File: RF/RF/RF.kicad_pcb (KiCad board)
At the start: 4 copper layers, 72.5 x 72.5 mm, 90 parts, among them IC201 CC1110F16RHHR, IC401 PE4250MLI-Z, IC501 RFFM6406SR, IC701 23K256-I_SN, IC702 SST25VF512A-33-4C-SAE, J101 Conn_Coaxial, J201 Conn_01x02, J601 Conn_01x02, J602 Conn_01x06, J603 Conn_02x05_Odd_Even, J801 ESQ-110-13-G-D, U301 0433BM15A0001, Y201 TG2520SMN 27.000M-MCGNNM3

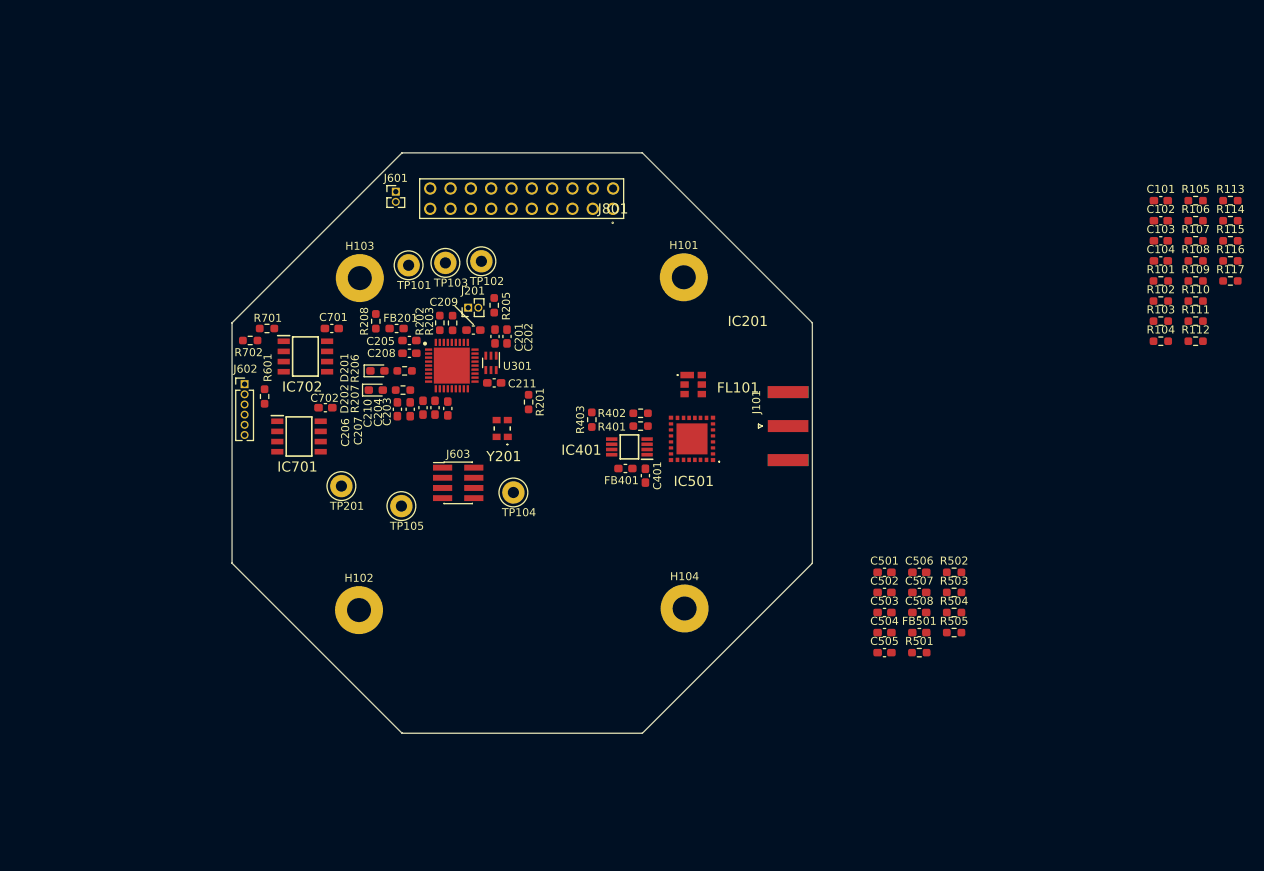
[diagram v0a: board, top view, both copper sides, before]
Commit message: layout rev 1.0
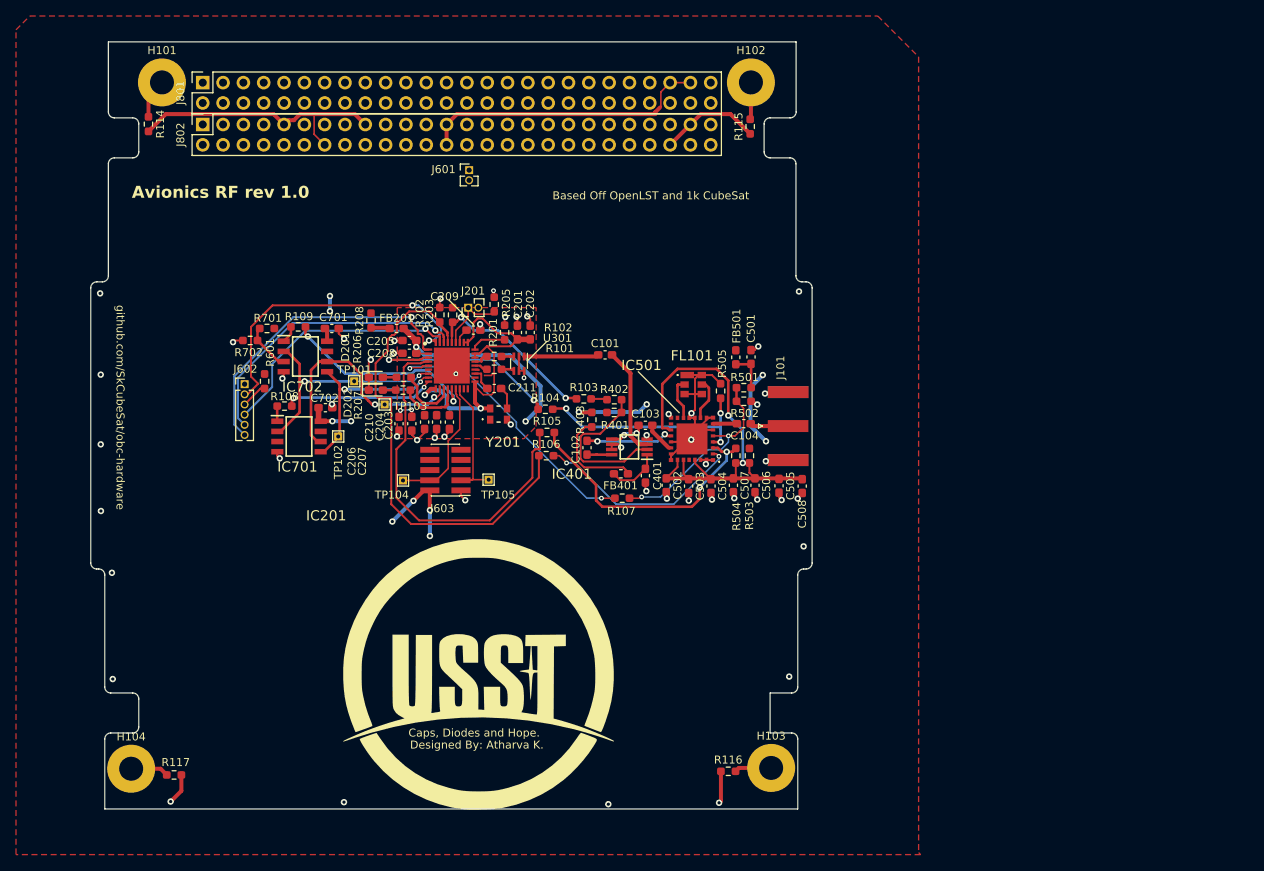
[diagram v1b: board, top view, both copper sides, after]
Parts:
- removed R110, R111, R112, R113: 0R, Resistor_SMD:R_0603_1608Metric_Pad0.98x0.95mm_HandSolder
- removed TP201: CC_SOC_2, TestPoint:TestPoint_Loop_D3.50mm_Drill1.4mm_Beaded
- added G***: LOGO, USST_logo:USST_logo, F.Cu at (108.5, 145.2)
- added G***: LOGO, USST_logo:USST_logo, B.Cu at (196.4, 139.0)
- added G***: LOGO, USST_logo:USST_logo, B.Cu at (207.5, 116.0)
- added G***: LOGO, USST_logo:USST_logo, B.Cu at (116.0, 116.7)
- added J802: Conn_02x26_Odd_Even, Connector_PinSocket_2.54mm:PinSocket_2x26_P2.54mm_Vertical, F.Cu at (74.1, 76.4)
- J603: footprint Connector_PinHeader_1.27mm:PinHeader_2x04_P1.27mm_Vertical_SMD -> Connector_PinHeader_1.27mm:PinHeader_2x05_P1.27mm_Vertical_SMD
- J801: value ESQ-110-13-G-D -> Conn_02x26_Odd_Even; footprint SamacSys_Parts:ESQ-110-Y-X-D -> Connector_PinSocket_2.54mm:PinSocket_2x26_P2.54mm_Vertical
- TP101, TP102, TP103, TP104, TP105: footprint TestPoint:TestPoint_Loop_D3.50mm_Drill1.4mm_Beaded -> TestPoint:TestPoint_THTPad_1.0x1.0mm_Drill0.5mm
- moved R117 145.8 mm to (70.5, 157.7), turned to 180 degrees
- moved R114 135.8 mm to (67.3, 76.4), turned to 90 degrees
- moved R108 115.3 mm to (84.3, 111.6), turned to 180 degrees
- moved R109 112.3 mm to (86.0, 101.7), turned to 180 degrees
- moved R116 89.5 mm to (139.8, 157.3)
- moved R106 86.3 mm to (117.0, 117.8)
- moved R105 86.1 mm to (117.1, 114.9)
- moved R101 84.1 mm to (110.5, 107.0)
- moved R102 83.6 mm to (110.5, 105.4)
- moved H102 82.2 mm to (142.6, 71.1)
- moved H103 80.0 mm to (145.1, 156.8)
- moved R107 78.6 mm to (126.5, 123.1)
- moved R104 77.4 mm to (116.9, 112.0)
- moved C102 77.1 mm to (122.1, 116.8), turned to 90 degrees
- moved R103 72.8 mm to (121.7, 110.7)
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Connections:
- IC201 pad 20: Net-(IC201-XOSC_Q2) -> unconnected-(IC201-XOSC_Q2-Pad20)
- J602 pad 2: /Connectors/UART0_RTS -> /CC1110/UART0_RTS
- J602 pad 4: /Connectors/UART0_RX -> /CC1110/UART0_RX
- J602 pad 5: /Connectors/UART0_TX -> /CC1110/UART0_TX
- J602 pad 6: /Connectors/UART0_CTS -> /CC1110/UART0_CTS
- J801 pad 1: /Standard Connector/GPIO_6 -> unconnected-(J801-Pin_1-Pad1)
- J801 pad 10: +5V -> unconnected-(J801-Pin_10-Pad10)
- J801 pad 11: /Standard Connector/GPIO_1 -> unconnected-(J801-Pin_11-Pad11)
- J801 pad 12: GND -> unconnected-(J801-Pin_12-Pad12)
- J801 pad 13: GND -> unconnected-(J801-Pin_13-Pad13)
- J801 pad 14: +3.3V -> unconnected-(J801-Pin_14-Pad14)
- J801 pad 15: /Standard Connector/CANL -> unconnected-(J801-Pin_15-Pad15)
- J801 pad 16: GND -> unconnected-(J801-Pin_16-Pad16)
- J801 pad 17: /Standard Connector/CANH -> unconnected-(J801-Pin_17-Pad17)
- J801 pad 18: +3.3V -> unconnected-(J801-Pin_18-Pad18)
- J801 pad 19: GND -> unconnected-(J801-Pin_19-Pad19)
- J801 pad 2: VBUS -> unconnected-(J801-Pin_2-Pad2)
- J801 pad 20: GND -> unconnected-(J801-Pin_20-Pad20)
- J801 pad 3: /Standard Connector/GPIO_5 -> unconnected-(J801-Pin_3-Pad3)
- J801 pad 4: GND -> unconnected-(J801-Pin_4-Pad4)
- J801 pad 5: /Standard Connector/GPIO_4 -> unconnected-(J801-Pin_5-Pad5)
- J801 pad 6: +5V -> unconnected-(J801-Pin_6-Pad6)
- J801 pad 7: /Standard Connector/GPIO_3 -> unconnected-(J801-Pin_7-Pad7)
- J801 pad 8: GND -> unconnected-(J801-Pin_8-Pad8)
- J801 pad 9: /Standard Connector/GPIO_2 -> unconnected-(J801-Pin_9-Pad9)
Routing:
- net GND: track 0.00 -> 135.8 mm, vias 0 -> 54
- net +3.3VA: track 0.00 -> 77.0 mm, vias 0 -> 6
- net Net-(IC501-VCC_RX): track 0.00 -> 70.8 mm, vias 0 -> 2
- net /CC1110/LST_TX_MODE: track 0.00 -> 59.7 mm
- net /CC1110/RF_EN: track 0.00 -> 47.0 mm
- net +3.3V: track 0.00 -> 41.5 mm, vias 0 -> 12
- net /CC1110/UART0_RTS: track 0.00 -> 39.2 mm, vias 0 -> 2
- net /CC1110/UART0_CTS: track 0.00 -> 38.5 mm, vias 0 -> 1
- net +5V: track 0.00 -> 36.7 mm
- net /CC1110/UART0_TX: track 0.00 -> 36.3 mm, vias 0 -> 1
- net /CC1110/AIN0: track 0.00 -> 35.5 mm, vias 0 -> 2
- net /RF Front End/RF_EN: track 0.00 -> 34.9 mm, vias 0 -> 2
- net /CC1110/UART0_RX: track 0.00 -> 31.7 mm, vias 0 -> 1
- net /SCK: track 0.00 -> 31.1 mm, vias 0 -> 2
- net /MISO: track 0.00 -> 29.0 mm, vias 0 -> 2
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- added copper zone on F.Cu, net +3.3V
- added copper zone on F.Cu, net +3.3VA
- added copper zone on In1.Cu, net GND
- added copper zone on In2.Cu, net GND
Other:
- board size 72.5 x 72.5 mm -> 90.2 x 95.9 mm
- board text added: "Avionics"
- board text added: "Avionics RF rev 1.0"
- board text added: "Based Off OpenLST and 1k CubeSat"
- board text added: "Caps, Diodes and Hope."
- board text added: "Designed By: Atharva K."
- board text added: "May 22, 2023"
- board text added: "RADSAT-SK 2 CubeSat OBC POC rev 1.0 By: Atharva K."
- board text added: "RF board rev. A"
- board text added: "github.com/SkCubeSat/obc-hardware"
